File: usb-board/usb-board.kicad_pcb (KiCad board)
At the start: 2 copper layers, 49.5 x 24.1 mm, 19 parts, among them J101 Conn_01x04_MountingPin, J102 USB_C_2.0, J103 Battery_Conn, SW101 PCM13SMTR, U101 MCP73831-2-OT

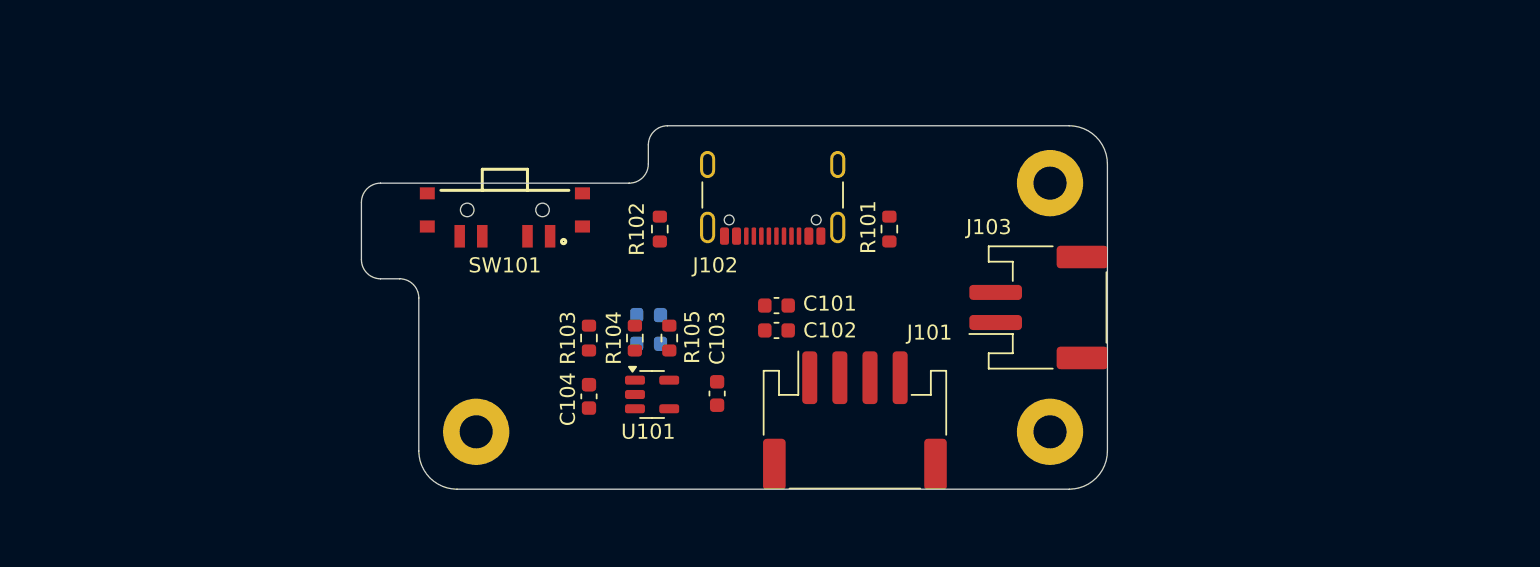
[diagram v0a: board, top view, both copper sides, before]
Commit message: revision 1 and 2 added
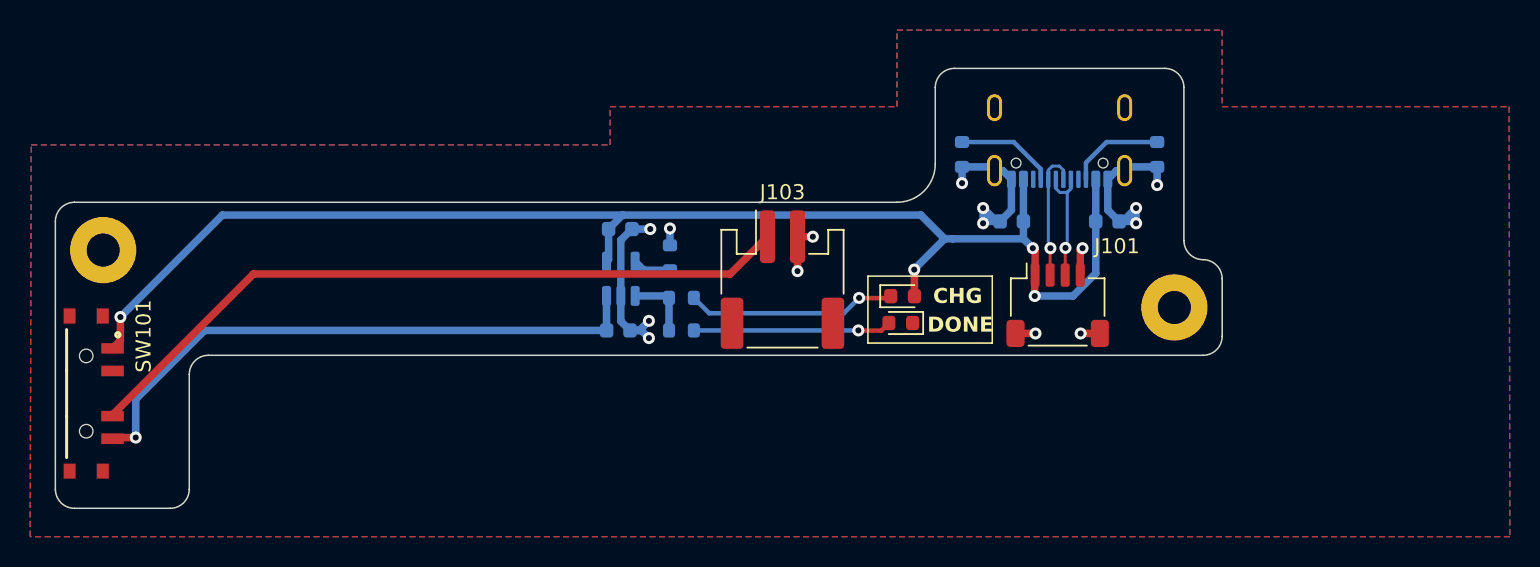
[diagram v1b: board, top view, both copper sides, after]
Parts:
- removed the H102 at (85.1, 34.3)
- C101, C102, C103, C104, J102, R101, R102, R103, R104, U101: moved to B.Cu
- D101, D102: moved to F.Cu
- J101: footprint Connector_JST:JST_PH_S4B-PH-SM4-TB_1x04-1MP_P2.00mm_Horizontal -> Connector_JST:JST_SH_SM04B-SRSS-TB_1x04-1MP_P1.00mm_Horizontal
- R105: value 5k -> 5.1k; moved to B.Cu
- moved R102 33.4 mm to (92.2, 32.4), turned to -90 degrees
- moved SW101 30.4 mm to (21.1, 48.3), turned to -90 degrees
- moved H102 27.5 mm to (22.2, 38.7)
- moved C102 23.1 mm to (88.9, 36.8), turned to 0 degrees
- moved J102 19.4 mm to (85.7, 30.4), turned to 0 degrees
- moved J103 17.1 mm to (67.3, 40.7), turned to 0 degrees
- moved D101 16.9 mm to (75.3, 41.8)
- moved D102 16.8 mm to (75.2, 43.6), turned to 180 degrees
- moved C101 16.6 mm to (82.5, 36.8)
- moved J101 15.5 mm to (85.6, 42.4)
- moved C103 12.7 mm to (56.6, 37.3), turned to 0 degrees
- moved H101 11.7 mm to (93.3, 42.5)
- moved U101 7.96 mm to (56.6, 40.6), turned to 90 degrees
- moved R101 6.92 mm to (79.2, 32.4), turned to -90 degrees
- moved R103 6.69 mm to (60.6, 41.9), turned to 180 degrees
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- renumbered H104 to H102
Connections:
- SW101 pad 1: unconnected-(SW101-Pad1) -> VCC
- SW101 pad 2: Net-(U101-V_{BAT}) -> unconnected-(SW101-Pad2)
- SW101 pad 4: VCC -> Net-(U101-V_{BAT})
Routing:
- net VCC: track 0.00 -> 92.9 mm, vias 0 -> 4
- net Net-(J103-Pin_1): track 0.00 -> 48.5 mm
- net GND: track 0.00 -> 43.5 mm, vias 0 -> 15
- net Net-(U101-V_{BAT}): track 0.00 -> 39.6 mm, vias 0 -> 1
- net Net-(D101-K): track 0.00 -> 14.0 mm, vias 0 -> 1
- net Net-(D102-A): track 0.00 -> 13.2 mm, vias 0 -> 1
- net USB_D+: track 0.00 -> 8.97 mm, vias 0 -> 1
- net USB_D-: track 0.00 -> 8.86 mm, vias 0 -> 1
- net Net-(J102-CC1): track 0.00 -> 6.65 mm
- net Net-(J102-CC2): track 0.00 -> 6.40 mm
- net Net-(U101-STAT): track 0.00 -> 4.46 mm
- net Net-(U101-PROG): track 0.00 -> 2.55 mm
- added copper zone on B.Cu, net GND
- added copper zone on F.Cu, net GND
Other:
- board size 49.5 x 24.1 mm -> 77.5 x 29.2 mm
